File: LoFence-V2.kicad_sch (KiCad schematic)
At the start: 58 parts, among them J1 DEBUG LED, J101 Fence+, J102 Fence-, J2 ISP, J3 DEBUG MCU, J4 DEBUG LA, SW1 RESET, U1 TPS63051RMW, U2 TLV9062, U3 ATmega328PB-AU, U4 LA66, Y1 32768 Hz

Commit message: fix part numbers
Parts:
- C1, C2, C3, C4: JLCPCB Part # C13585 -> (none)
- C10, C11, C12, C5, C6, C7, C8, C9: JLCPCB Part # C49678 -> (none)
- U1: JLCPCB Part # (none) -> C139412
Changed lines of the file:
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@@
       (effects (font (size 1.27 1.27)) hide)
     )
-    (property "JLCPCB Part #" "C49678" (at 252.73 55.88 0)
+    (property "JLCPCB Part #" "" (at 252.73 55.88 0)
       (effects (font (size 1.27 1.27)) hide)
     )
@@
       (effects (font (size 1.27 1.27)) hide)
     )
-    (property "JLCPCB Part #" "C49678" (at 76.2 69.85 0)
+    (property "JLCPCB Part #" "" (at 76.2 69.85 0)
       (effects (font (size 1.27 1.27)) hide)
     )
@@
       (effects (font (size 1.27 1.27)) hide)
     )
-    (property "JLCPCB Part #" "C13585" (at 127 33.02 0)
+    (property "JLCPCB Part #" "" (at 127 33.02 0)
       (effects (font (size 1.27 1.27)) hide)
     )
@@
       (effects (font (size 1.27 1.27)) hide)
     )
-    (property "JLCPCB Part #" "C49678" (at 76.2 113.03 0)
+    (property "JLCPCB Part #" "" (at 76.2 113.03 0)
       (effects (font (size 1.27 1.27)) hide)
     )
@@
       (effects (font (size 1.27 1.27)) hide)
     )
-    (property "JLCPCB Part #" "C49678" (at 104.14 90.17 0)
+    (property "JLCPCB Part #" "" (at 104.14 90.17 0)
       (effects (font (size 1.27 1.27)) hide)
     )
@@
       (effects (font (size 1.27 1.27)) hide)
     )
-    (property "JLCPCB Part #" "C49678" (at 245.11 86.36 0)
+    (property "JLCPCB Part #" "" (at 245.11 86.36 0)
       (effects (font (size 1.27 1.27)) hide)
     )
@@
       (effects (font (size 1.27 1.27)) hide)
     )
-    (property "JLCPCB Part #" "C13585" (at 210.82 30.48 0)
+    (property "JLCPCB Part #" "" (at 210.82 30.48 0)
       (effects (font (size 1.27 1.27)) hide)
     )
@@
       (effects (font (size 1.27 1.27)) hide)
     )
-    (property "JLCPCB Part #" "C13585" (at 199.39 30.48 0)
+    (property "JLCPCB Part #" "" (at 199.39 30.48 0)
       (effects (font (size 1.27 1.27)) hide)
     )
@@
       (effects (font (size 1.27 1.27)) hide)
     )
-    (property "JLCPCB Part #" "C49678" (at 40.64 132.08 0)
+    (property "JLCPCB Part #" "" (at 40.64 132.08 0)
       (effects (font (size 1.27 1.27)) hide)
     )
@@
       (effects (font (size 1.27 1.27)) hide)
     )
-    (property "JLCPCB Part #" "C49678" (at 160.02 148.59 0)
+    (property "JLCPCB Part #" "" (at 160.02 148.59 0)
       (effects (font (size 1.27 1.27)) hide)
     )
@@
       (effects (font (size 1.27 1.27)) hide)
     )
-    (property "JLCPCB Part #" "C49678" (at 166.37 148.59 0)
+    (property "JLCPCB Part #" "" (at 166.37 148.59 0)
       (effects (font (size 1.27 1.27)) hide)
     )
@@
     )
     (property "TME Order #" "" (at 158.75 36.83 0)
+      (effects (font (size 1.27 1.27)) hide)
+    )
+    (property "JLCPCB Part #" "C139412" (at 158.75 36.83 0)
       (effects (font (size 1.27 1.27)) hide)
     )
@@
       (effects (font (size 1.27 1.27)) hide)
     )
-    (property "JLCPCB Part #" "C13585" (at 177.8 41.91 0)
-      (effects (font (size 1.27 1.27)) hide)
-    )
+    (property "JLCPCB Part #" "" (at 177.8 41.91 0)
+      (effects (font (size 1.27 1.27)) hide)
+    )

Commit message: add TME order numbers
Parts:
- R2: TME Order # (none) -> MGR0.25W-1M
- R3: TME Order # (none) -> RC0805FR-075K76L
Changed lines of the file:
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@@
       (effects (font (size 1.27 1.27)) hide)
     )
-    (property "TME Order #" "" (at 45.72 21.59 0)
+    (property "TME Order #" "MGR0.25W-1M" (at 45.72 21.59 0)
       (effects (font (size 1.27 1.27)) hide)
     )
@@
       (effects (font (size 1.27 1.27)) hide)
     )
-    (property "TME Order #" "" (at 55.88 21.59 0)
+    (property "TME Order #" "RC0805FR-075K76L" (at 55.88 21.59 0)
       (effects (font (size 1.27 1.27)) hide)
     )

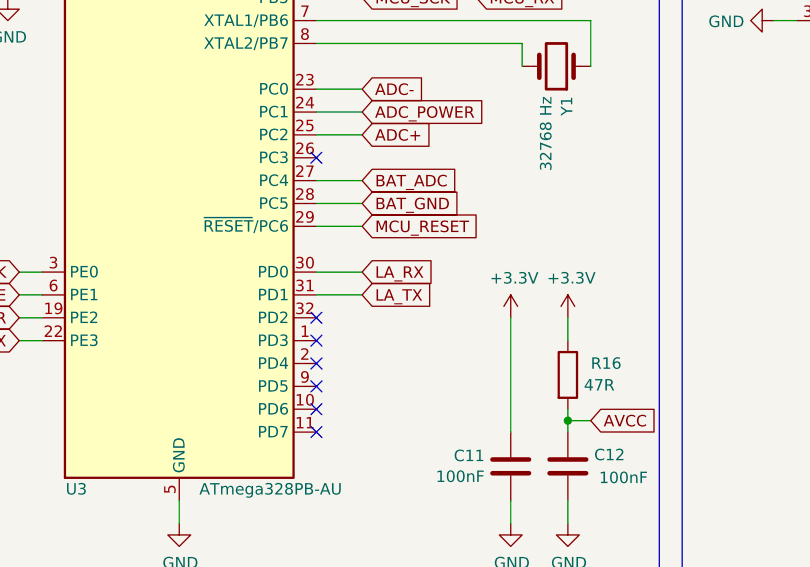
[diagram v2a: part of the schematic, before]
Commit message: fix TA66 rx and tx
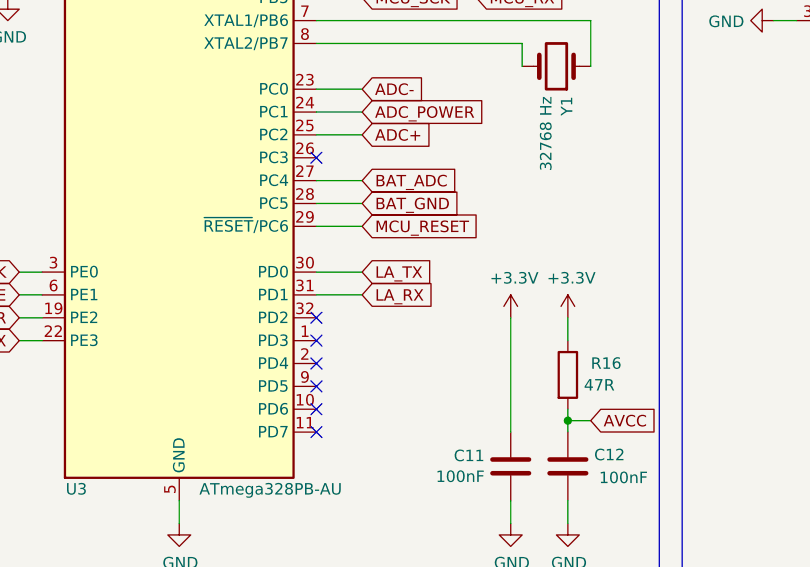
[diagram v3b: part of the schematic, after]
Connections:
- net LA_RX: now also U3.31 (PD1); no longer U3.30 (PD0)
- net LA_TX: now also U3.30 (PD0); no longer U3.31 (PD1)
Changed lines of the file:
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@@
     )
   )
-  (global_label "LA_TX" (shape input) (at 143.51 129.54 0) (fields_autoplaced)
+  (global_label "LA_RX" (shape input) (at 143.51 129.54 0) (fields_autoplaced)
     (effects (font (size 1.27 1.27)) (justify left))
-    (property "Intersheetrefs" "${INTERSHEET_REFS}" (at 151.1024 129.54 0)
+    (property "Intersheetrefs" "${INTERSHEET_REFS}" (at 151.4048 129.54 0)
       (effects (font (size 1.27 1.27)) (justify left) hide)
     )
@@
     )
   )
-  (global_label "LA_RX" (shape input) (at 143.51 127 0) (fields_autoplaced)
+  (global_label "LA_TX" (shape input) (at 143.51 127 0) (fields_autoplaced)
     (effects (font (size 1.27 1.27)) (justify left))
-    (property "Intersheetrefs" "${INTERSHEET_REFS}" (at 151.4048 127 0)
+    (property "Intersheetrefs" "${INTERSHEET_REFS}" (at 151.1024 127 0)
       (effects (font (size 1.27 1.27)) (justify left) hide)
     )
